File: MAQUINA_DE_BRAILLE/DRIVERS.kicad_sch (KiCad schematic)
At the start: 26 parts, among them J1 Screw_Terminal_01x04, J2 Screw_Terminal_01x04, U2 DRV8825PWPR, U3 DRV8825PWPR

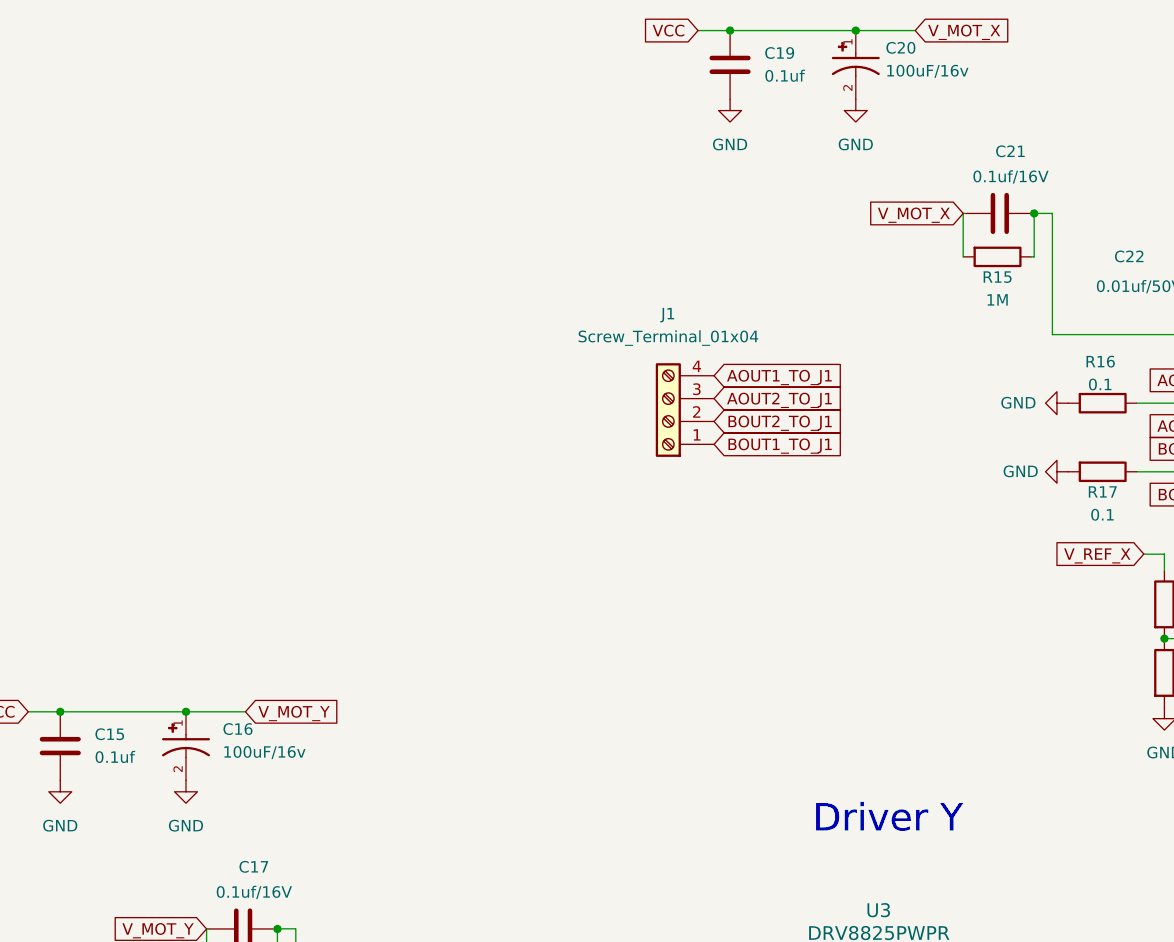
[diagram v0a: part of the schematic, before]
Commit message: LAST UPDATE
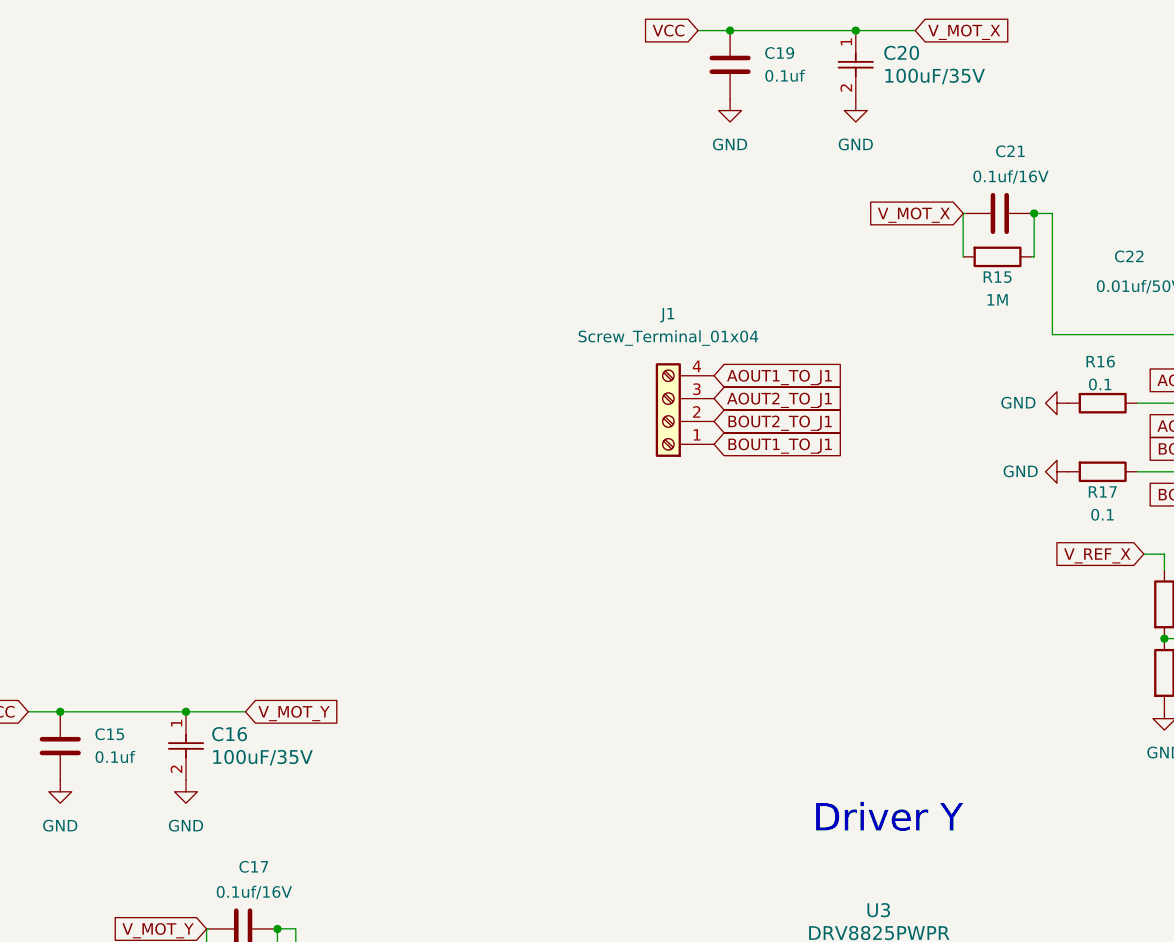
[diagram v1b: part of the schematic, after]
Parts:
- removed C16, C20: 100uF/16v, EEETC1C101XV:CAP_EEETC1C101XV, symbol EEETC1C101XV:EEETC1C101XV
- added C16, C20: 100uF/35V, 865080545012:CAP_WCAP-ASLI_06p3X07p7_WRE, symbol 865080545012:865080545012
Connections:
- net GND: now also C16.2, C20.2
- net VCC: now also C16.1, C20.1
